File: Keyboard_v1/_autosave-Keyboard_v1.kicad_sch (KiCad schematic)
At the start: 16 parts, among them SW1 SW_Push, U1 ATmega32U4-A, Y1 16MHz

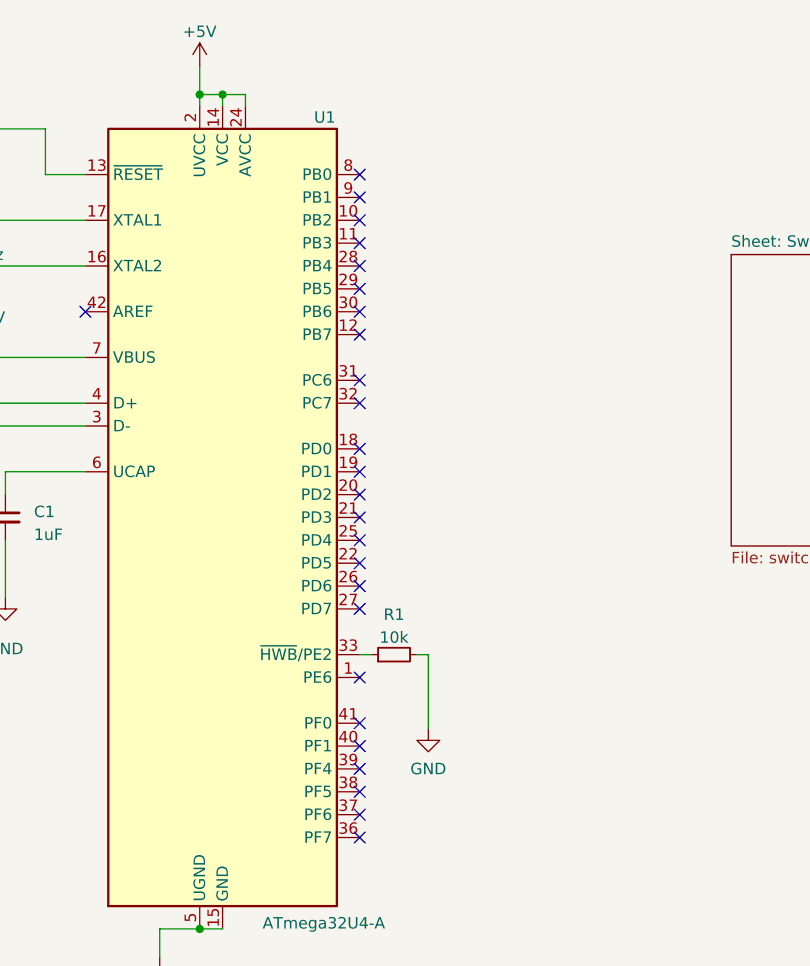
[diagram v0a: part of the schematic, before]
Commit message: all rows and cols connected to MCU
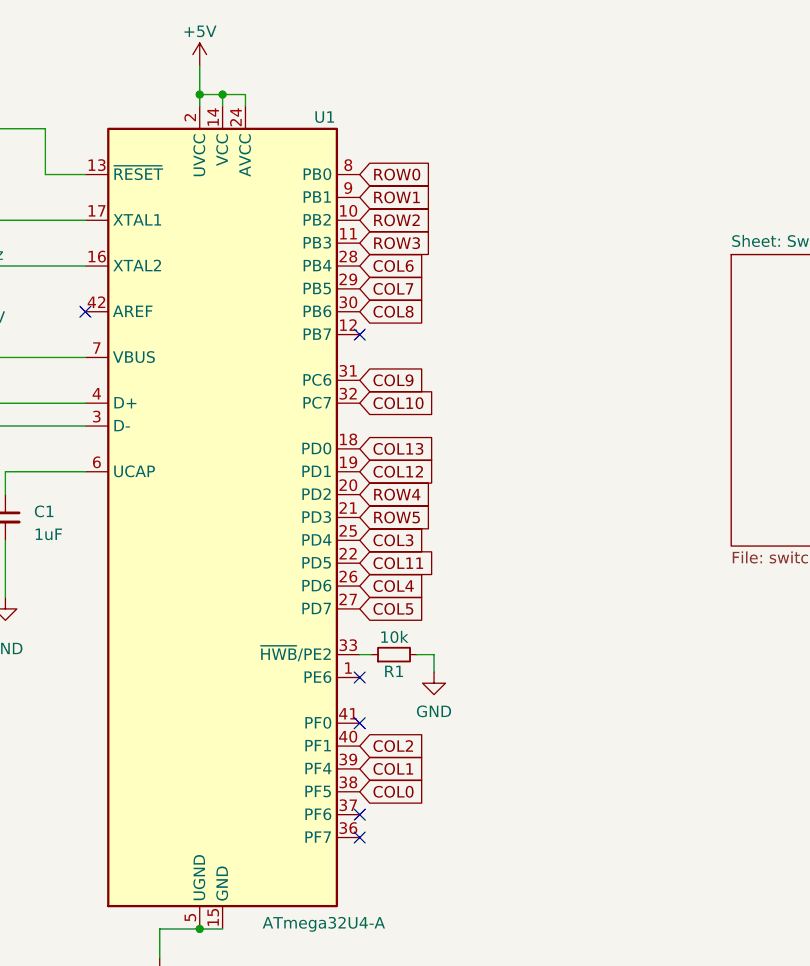
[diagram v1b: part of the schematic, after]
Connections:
- net ROW2: now reaches U1.10 (PB2)
- net ROW3: now reaches U1.11 (PB3)
- net COL13: now reaches U1.18 (PD0)
- net COL12: now reaches U1.19 (PD1)
- net ROW4: now reaches U1.20 (PD2)
- net ROW5: now reaches U1.21 (PD3)
- net COL11: now reaches U1.22 (PD5)
- net COL3: now reaches U1.25 (PD4)
- net COL4: now reaches U1.26 (PD6)
- net COL5: now reaches U1.27 (PD7)
- net COL6: now reaches U1.28 (PB4)
- net COL7: now reaches U1.29 (PB5)
- net COL8: now reaches U1.30 (PB6)
- net COL9: now reaches U1.31 (PC6)
- net COL10: now reaches U1.32 (PC7)
- net COL0: now reaches U1.38 (PF5)
- net COL1: now reaches U1.39 (PF4)
- net COL2: now reaches U1.40 (PF1)
- net ROW0: now reaches U1.8 (PB0)
- net ROW1: now reaches U1.9 (PB1)
- no-connect marks 26 -> 6
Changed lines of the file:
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@@
   (junction (at 125.095 60.96) (diameter 0) (color 0 0 0 0)
   )
-  (no_connect (at 175.26 83.82))
   (no_connect (at 175.26 106.68))
   (no_connect (at 144.78 66.04))
-  (no_connect (at 175.26 66.04))
-  (no_connect (at 175.26 96.52))
-  (no_connect (at 175.26 63.5))
   (no_connect (at 175.26 121.92))
-  (no_connect (at 175.26 99.06))
-  (no_connect (at 175.26 116.84))
-  (no_connect (at 175.26 50.8))
-  (no_connect (at 175.26 119.38))
-  (no_connect (at 175.26 58.42))
-  (no_connect (at 175.26 55.88))
-  (no_connect (at 175.26 114.3))
-  (no_connect (at 175.26 53.34))
-  (no_connect (at 175.26 73.66))
-  (no_connect (at 175.26 93.98))
-  (no_connect (at 175.26 81.28))
-  (no_connect (at 175.26 86.36))
   (no_connect (at 175.26 111.76))
-  (no_connect (at 175.26 60.96))
   (no_connect (at 175.26 124.46))
   (no_connect (at 175.26 68.58))
-  (no_connect (at 175.26 88.9))
-  (no_connect (at 175.26 91.44))
-  (no_connect (at 175.26 76.2))
   (wire (pts (xy 162.56 41.91) (xy 162.56 43.18))
     (stroke (width 0) (type default))
@@
     (stroke (width 0) (type default))
   )
-  (wire (pts (xy 182.88 104.14) (xy 182.88 112.395))
+  (wire (pts (xy 183.515 104.14) (xy 183.515 106.045))
     (stroke (width 0) (type default))
   )
@@
     (stroke (width 0) (type default))
   )
-  (wire (pts (xy 181.61 104.14) (xy 182.88 104.14))
+  (wire (pts (xy 181.61 104.14) (xy 183.515 104.14))
     (stroke (width 0) (type default))
   )
@@
     (effects (font (size 1.27 1.27)) (justify left bottom))
   )
+  (global_label "COL4" (shape input) (at 175.26 96.52 0) (fields_autoplaced)
+    (effects (font (size 1.27 1.27)) (justify left))
+    (property "Intersheetrefs" "${INTERSHEET_REFS}" (at 183.0039 96.52 0)
+      (effects (font (size 1.27 1.27)) (justify left) hide)
+    )
+  )
+  (global_label "COL0" (shape input) (at 175.26 119.38 0) (fields_autoplaced)
+    (effects (font (size 1.27 1.27)) (justify left))
+    (property "Intersheetrefs" "${INTERSHEET_REFS}" (at 183.0039 119.38 0)
+      (effects (font (size 1.27 1.27)) (justify left) hide)
+    )
+  )
+  (global_label "COL8" (shape input) (at 175.26 66.04 0) (fields_autoplaced)
+    (effects (font (size 1.27 1.27)) (justify left))
+    (property "Intersheetrefs" "${INTERSHEET_REFS}" (at 183.0039 66.04 0)
+      (effects (font (size 1.27 1.27)) (justify left) hide)
+    )
+  )
+  (global_label "COL10" (shape input) (at 175.26 76.2 0) (fields_autoplaced)
+    (effects (font (size 1.27 1.27)) (justify left))
+    (property "Intersheetrefs" "${INTERSHEET_REFS}" (at 184.2134 76.2 0)
+      (effects (font (size 1.27 1.27)) (justify left) hide)
+    )
+  )
   (global_label "D+" (shape input) (at 70.485 151.13 0) (fields_autoplaced)
     (effects (font (size 1.27 1.27)) (justify left))
@@
     )
   )
+  (global_label "COL12" (shape input) (at 175.26 83.82 0) (fields_autoplaced)
+    (effects (font (size 1.27 1.27)) (justify left))
+    (property "Intersheetrefs" "${INTERSHEET_REFS}" (at 184.2134 83.82 0)
+      (effects (font (size 1.27 1.27)) (justify left) hide)
+    )
+  )
+  (global_label "COL5" (shape input) (at 175.26 99.06 0) (fields_autoplaced)
+    (effects (font (size 1.27 1.27)) (justify left))
+    (property "Intersheetrefs" "${INTERSHEET_REFS}" (at 183.0039 99.06 0)
+      (effects (font (size 1.27 1.27)) (justify left) hide)
+    )
+  )
   (global_label "D-" (shape input) (at 70.485 148.59 0) (fields_autoplaced)
     (effects (font (size 1.27 1.27)) (justify left))
     (property "Intersheetrefs" "${INTERSHEET_REFS}" (at 76.2332 148.59 0)
+      (effects (font (size 1.27 1.27)) (justify left) hide)
+    )
+  )
+  (global_label "ROW0" (shape input) (at 175.26 50.8 0) (fields_autoplaced)
+    (effects (font (size 1.27 1.27)) (justify left))
+    (property "Intersheetrefs" "${INTERSHEET_REFS}" (at 183.4272 50.8 0)
+      (effects (font (size 1.27 1.27)) (justify left) hide)
+    )
+  )
+  (global_label "COL7" (shape input) (at 175.26 63.5 0) (fields_autoplaced)
+    (effects (font (size 1.27 1.27)) (justify left))
+    (property "Intersheetrefs" "${INTERSHEET_REFS}" (at 183.0039 63.5 0)
+      (effects (font (size 1.27 1.27)) (justify left) hide)
+    )
+  )
+  (global_label "ROW2" (shape input) (at 175.26 55.88 0) (fields_autoplaced)
+    (effects (font (size 1.27 1.27)) (justify left))
+    (property "Intersheetrefs" "${INTERSHEET_REFS}" (at 183.4272 55.88 0)
+      (effects (font (size 1.27 1.27)) (justify left) hide)
+    )
+  )
+  (global_label "ROW4" (shape input) (at 175.26 86.36 0) (fields_autoplaced)
+    (effects (font (size 1.27 1.27)) (justify left))
+    (property "Intersheetrefs" "${INTERSHEET_REFS}" (at 183.4272 86.36 0)
+      (effects (font (size 1.27 1.27)) (justify left) hide)
+    )
+  )
+  (global_label "COL13" (shape input) (at 175.26 81.28 0) (fields_autoplaced)
+    (effects (font (size 1.27 1.27)) (justify left))
+    (property "Intersheetrefs" "${INTERSHEET_REFS}" (at 184.2134 81.28 0)
+      (effects (font (size 1.27 1.27)) (justify left) hide)
+    )
+  )
+  (global_label "COL1" (shape input) (at 175.26 116.84 0) (fields_autoplaced)
+    (effects (font (size 1.27 1.27)) (justify left))
+    (property "Intersheetrefs" "${INTERSHEET_REFS}" (at 183.0039 116.84 0)
+      (effects (font (size 1.27 1.27)) (justify left) hide)
+    )
+  )
+  (global_label "COL9" (shape input) (at 175.26 73.66 0) (fields_autoplaced)
+    (effects (font (size 1.27 1.27)) (justify left))
+    (property "Intersheetrefs" "${INTERSHEET_REFS}" (at 183.0039 73.66 0)
+      (effects (font (size 1.27 1.27)) (justify left) hide)
+    )
+  )
+  (global_label "COL3" (shape input) (at 175.26 91.44 0) (fields_autoplaced)
+    (effects (font (size 1.27 1.27)) (justify left))
+    (property "Intersheetrefs" "${INTERSHEET_REFS}" (at 183.0039 91.44 0)
       (effects (font (size 1.27 1.27)) (justify left) hide)
     )
@@
     (property "Intersheetrefs" "${INTERSHEET_REFS}" (at 101.5668 76.2 0)
       (effects (font (size 1.27 1.27)) (justify right) hide)
+    )
+  )
+  (global_label "COL2" (shape input) (at 175.26 114.3 0) (fields_autoplaced)
+    (effects (font (size 1.27 1.27)) (justify left))
+    (property "Intersheetrefs" "${INTERSHEET_REFS}" (at 183.0039 114.3 0)
+      (effects (font (size 1.27 1.27)) (justify left) hide)
+    )
+  )
+  (global_label "ROW1" (shape input) (at 175.26 53.34 0) (fields_autoplaced)
+    (effects (font (size 1.27 1.27)) (justify left))
+    (property "Intersheetrefs" "${INTERSHEET_REFS}" (at 183.4272 53.34 0)
+      (effects (font (size 1.27 1.27)) (justify left) hide)
+    )
+  )
+  (global_label "ROW5" (shape input) (at 175.26 88.9 0) (fields_autoplaced)
+    (effects (font (size 1.27 1.27)) (justify left))
+    (property "Intersheetrefs" "${INTERSHEET_REFS}" (at 183.4272 88.9 0)
+      (effects (font (size 1.27 1.27)) (justify left) hide)
+    )
+  )
+  (global_label "COL6" (shape input) (at 175.26 60.96 0) (fields_autoplaced)
+    (effects (font (size 1.27 1.27)) (justify left))
+    (property "Intersheetrefs" "${INTERSHEET_REFS}" (at 183.0039 60.96 0)
+      (effects (font (size 1.27 1.27)) (justify left) hide)
+    )
+  )
+  (global_label "COL11" (shape input) (at 175.26 93.98 0) (fields_autoplaced)
+    (effects (font (size 1.27 1.27)) (justify left))
+    (property "Intersheetrefs" "${INTERSHEET_REFS}" (at 184.2134 93.98 0)
+      (effects (font (size 1.27 1.27)) (justify left) hide)
+    )
+  )
+  (global_label "ROW3" (shape input) (at 175.26 58.42 0) (fields_autoplaced)
+    (effects (font (size 1.27 1.27)) (justify left))
+    (property "Intersheetrefs" "${INTERSHEET_REFS}" (at 183.4272 58.42 0)
+      (effects (font (size 1.27 1.27)) (justify left) hide)
     )
   )
@@
   )
   (symbol (lib_id "Device:R_Small") (at 179.07 104.14 90) (unit 1)
-    (in_bom yes) (on_board yes) (dnp no) (fields_autoplaced)
-    (property "Reference" "R1" (at 179.07 99.695 90)
+    (in_bom yes) (on_board yes) (dnp no)
+    (property "Reference" "R1" (at 179.07 106.045 90)
       (effects (font (size 1.27 1.27)))
     )
@@
     )
   )
-  (symbol (lib_id "power:GND") (at 182.88 112.395 0) (unit 1)
-    (in_bom yes) (on_board yes) (dnp no) (fields_autoplaced)
-    (property "Reference" "#PWR03" (at 182.88 118.745 0)
-      (effects (font (size 1.27 1.27)) hide)
-    )
-    (property "Value" "GND" (at 182.88 116.84 0)
-      (effects (font (size 1.27 1.27)))
-    )
-    (property "Footprint" "" (at 182.88 112.395 0)
-      (effects (font (size 1.27 1.27)) hide)
-    )
-    (property "Datasheet" "" (at 182.88 112.395 0)
-      (effects (font (size 1.27 1.27)) hide)
-    )
+  (symbol (lib_id "power:GND") (at 183.515 106.045 0) (unit 1)
+    (in_bom yes) (on_board yes) (dnp no) (fields_autoplaced)
+    (property "Reference" "#PWR03" (at 183.515 112.395 0)
+      (effects (font (size 1.27 1.27)) hide)
+    )
+    (property "Value" "GND" (at 183.515 110.49 0)
+      (effects (font (size 1.27 1.27)))
+    )
+    (property "Footprint" "" (at 183.515 106.045 0)
+      (effects (font (size 1.27 1.27)) hide)
+    )
+    (property "Datasheet" "" (at 183.515 106.045 0)
+      (effects (font (size 1.27 1.27)) hide)
+    )
